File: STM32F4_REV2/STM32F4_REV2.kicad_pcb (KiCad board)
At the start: 4 copper layers, 50.8 x 50.7 mm, 70 parts, among them IC1 MP2359DJ-LF-Z, J1 Screw_Terminal_01x02, J2 SWD, J3 Conn_01x04, J4 Conn_01x04, J5 USB_B_Micro, J6 Conn_01x04, J7 Conn_01x04, J8 Conn_01x02, Q1 AO3401A, SW1 SW_SPDT, SW2 SW_Push, U1 STM32F405RGT6, U2 USBLC6-2SC6, Y1 16MHz

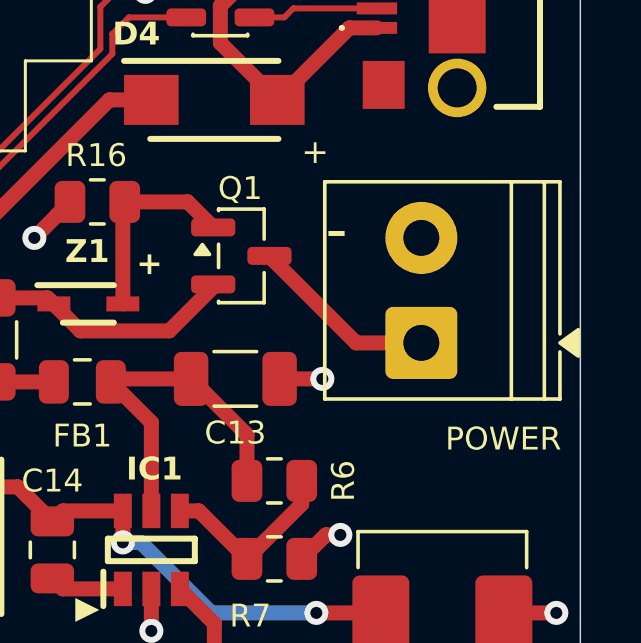
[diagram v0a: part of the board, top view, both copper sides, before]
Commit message: Modified'
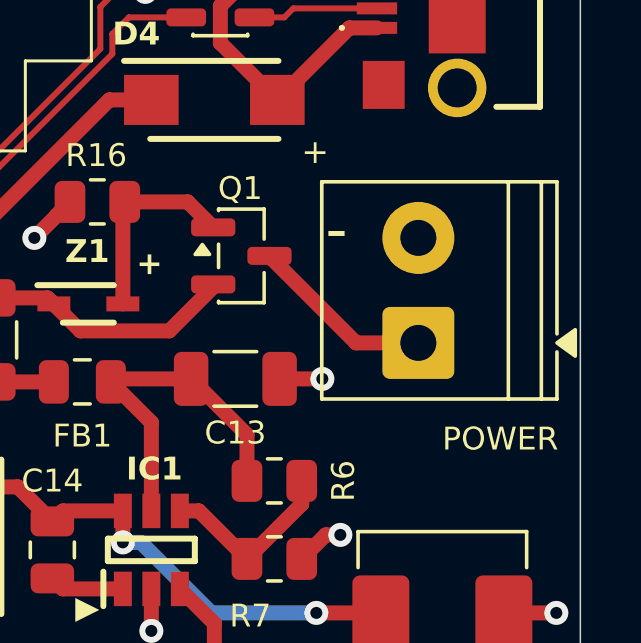
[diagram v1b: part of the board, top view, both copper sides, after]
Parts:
- moved J1 0.10 mm to (166.4, 102.6)
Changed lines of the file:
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@@
 	(footprint "TerminalBlock_Phoenix:TerminalBlock_Phoenix_PT-1,5-2-3.5-H_1x02_P3.50mm_Horizontal"
 		(layer "F.Cu")
-		(at 166.5 102.6 90)
+		(at 166.4 102.6 90)
 		(descr "Terminal Block Phoenix PT-1,5-2-3.5-H, 2 pins, pitch 3.5mm, size 7x7.6mm, drill diameter 1.2mm, pad diameter 2.4mm, ")
 		(tags "THT Terminal Block Phoenix PT-1,5-2-3.5-H pitch 3.5mm size 7x7.6mm drill 1.2mm pad 2.4mm")
@@
 	)
 	(segment
-		(start 161.5375 99.8)
-		(end 161.4375 99.7)
+		(start 164.325 102.6)
+		(end 161.5375 99.8125)
 		(width 0.5)
 		(layer "F.Cu")
@@
 	)
 	(segment
-		(start 166.5 102.6)
+		(start 166.4 102.6)
 		(end 164.325 102.6)
 		(width 0.5)
@@
 	)
 	(segment
-		(start 164.325 102.6)
-		(end 161.5375 99.8125)
+		(start 161.5375 99.8)
+		(end 161.4375 99.7)
 		(width 0.5)
 		(layer "F.Cu")
